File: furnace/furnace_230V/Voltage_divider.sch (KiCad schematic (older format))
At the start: 14 parts

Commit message: Add files via upload
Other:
- note added: "Input 230V voltage measurement circuit"
- note removed: "Input 230V voltage mesurement circuit"
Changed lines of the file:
@@
 $EndComp
 Text Notes 8850 2200 2    197  ~ 0
-Input 230V voltage mesurement circuit
+Input 230V voltage measurement circuit
 $Comp
 L Device:C C?

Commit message: Add files via upload
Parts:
- C15, C16, C17: renamed from C?; symbol Device:C -> furnace_230V-rescue:C-Device
- D4: renamed from D?; footprint (none) -> Diode_SMD:D_SMA-SMB_Universal_Handsoldering; symbol Device:D -> furnace_230V-rescue:D-Device
- D5: renamed from D?; symbol Diode:BAT54S -> furnace_230V-rescue:BAT54S-Diode
- D6: renamed from D?; footprint (none) -> Diode_SMD:D_SMA-SMB_Universal_Handsoldering; symbol Device:D_TVS -> furnace_230V-rescue:D_TVS-Device
- R10, R11, R12, R13, R14: renamed from R?; symbol Device:R -> furnace_230V-rescue:R-Device
- TP7, TP8, TP9: renamed from TP?; symbol Connector:TestPoint -> furnace_230V-rescue:TestPoint-Connector
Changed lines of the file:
@@
 $EndDescr
 $Comp
-L Device:R R?
+L furnace_230V-rescue:R-Device R?
 U 1 1 60AC3251
 P 4500 3650
 AR Path="/60AAE0B8/60AC3251" Ref="R?"  Part="1"
-AR Path="/60AAE4BD/60AC3251" Ref="R?"  Part="1"
-F 0 "R?" H 4570 3696 50  0000 L CNN
+AR Path="/60AAE4BD/60AC3251" Ref="R10"  Part="1"
+F 0 "R10" H 4570 3696 50  0000 L CNN
 F 1 "180k 0,25W 1%" H 4570 3605 50  0000 L CNN
 F 2 "" V 4430 3650 50  0001 C CNN
@@
 $EndComp
 $Comp
-L Device:R R?
+L furnace_230V-rescue:R-Device R?
 U 1 1 60AC39AB
 P 6150 4000
 AR Path="/60AAE0B8/60AC39AB" Ref="R?"  Part="1"
 AR Path="/60AAEC6C/60AC39AB" Ref="R?"  Part="1"
-AR Path="/60AAE4BD/60AC39AB" Ref="R?"  Part="1"
-F 0 "R?" V 6050 4000 50  0000 C CNN
+AR Path="/60AAE4BD/60AC39AB" Ref="R13"  Part="1"
+F 0 "R13" V 6050 4000 50  0000 C CNN
 F 1 "100" V 6250 4000 50  0000 C CNN
 F 2 "Resistor_SMD:R_0603_1608Metric_Pad1.05x0.95mm_HandSolder" V 6080 4000 50  0001 C CNN
@@
 $EndComp
 $Comp
-L Diode:BAT54S D?
+L furnace_230V-rescue:BAT54S-Diode D5
 U 1 1 60AC3BC9
 P 6700 3500
-F 0 "D?" V 6746 3588 50  0000 L CNN
+F 0 "D5" V 6746 3588 50  0000 L CNN
 F 1 "BAT54S" V 6655 3588 50  0000 L CNN
 F 2 "Package_TO_SOT_SMD:SOT-23" H 6775 3625 50  0001 L CNN
@@
 $EndComp
 $Comp
-L Device:D_TVS D?
+L furnace_230V-rescue:D_TVS-Device D6
 U 1 1 60AC5492
 P 7000 4150
-F 0 "D?" V 7050 4000 50  0000 C CNN
+F 0 "D6" V 7050 4000 50  0000 C CNN
 F 1 "D_TVS" V 6950 3950 50  0000 C CNN
-F 2 "" H 7000 4150 50  0001 C CNN
+F 2 "Diode_SMD:D_SMA-SMB_Universal_Handsoldering" H 7000 4150 50  0001 C CNN
 F 3 "~" H 7000 4150 50  0001 C CNN
 	1    7000 4150
@@
 $EndComp
 $Comp
-L Device:R R?
+L furnace_230V-rescue:R-Device R?
 U 1 1 60AC5A68
 P 7650 4000
 AR Path="/60AAE0B8/60AC5A68" Ref="R?"  Part="1"
 AR Path="/60AAEC6C/60AC5A68" Ref="R?"  Part="1"
-AR Path="/60AAE4BD/60AC5A68" Ref="R?"  Part="1"
-F 0 "R?" V 7550 4000 50  0000 C CNN
+AR Path="/60AAE4BD/60AC5A68" Ref="R14"  Part="1"
+F 0 "R14" V 7550 4000 50  0000 C CNN
 F 1 "1k" V 7750 4000 50  0000 C CNN
 F 2 "Resistor_SMD:R_0603_1608Metric_Pad1.05x0.95mm_HandSolder" V 7580 4000 50  0001 C CNN
@@
 $EndComp
 $Comp
-L Device:C C?
+L furnace_230V-rescue:C-Device C?
 U 1 1 60AC6425
 P 8000 4150
@@
 AR Path="/609CA6A8/60AE5653/60AC6425" Ref="C?"  Part="1"
 AR Path="/60AAC605/60AC6425" Ref="C?"  Part="1"
-AR Path="/60AAE4BD/60AC6425" Ref="C?"  Part="1"
-F 0 "C?" H 8115 4196 50  0000 L CNN
+AR Path="/60AAE4BD/60AC6425" Ref="C17"  Part="1"
+F 0 "C17" H 8115 4196 50  0000 L CNN
 F 1 "100" H 8115 4105 50  0000 L CNN
 F 2 "Capacitor_SMD:C_0603_1608Metric_Pad1.08x0.95mm_HandSolder" H 8038 4000 50  0001 C CNN
@@
 $EndComp
 $Comp
-L Connector:TestPoint TP?
+L furnace_230V-rescue:TestPoint-Connector TP?
 U 1 1 60ACD704
 P 5500 4000
@@
 AR Path="/609CA6A8/60AE5653/60ACD704" Ref="TP?"  Part="1"
 AR Path="/60AAC605/60ACD704" Ref="TP?"  Part="1"
-AR Path="/60AAE4BD/60ACD704" Ref="TP?"  Part="1"
-F 0 "TP?" H 5558 4118 50  0000 L CNN
+AR Path="/60AAE4BD/60ACD704" Ref="TP7"  Part="1"
+F 0 "TP7" H 5558 4118 50  0000 L CNN
 F 1 "TestPoint" H 5558 4027 50  0001 L CNN
 F 2 "" H 5700 4000 50  0001 C CNN
@@
 $EndComp
 $Comp
-L Connector:TestPoint TP?
+L furnace_230V-rescue:TestPoint-Connector TP?
 U 1 1 60ACD8BB
 P 5500 4500
@@
 AR Path="/609CA6A8/60AE5653/60ACD8BB" Ref="TP?"  Part="1"
 AR Path="/60AAC605/60ACD8BB" Ref="TP?"  Part="1"
-AR Path="/60AAE4BD/60ACD8BB" Ref="TP?"  Part="1"
-F 0 "TP?" H 5558 4618 50  0000 L CNN
+AR Path="/60AAE4BD/60ACD8BB" Ref="TP8"  Part="1"
+F 0 "TP8" H 5558 4618 50  0000 L CNN
 F 1 "TestPoint" H 5558 4527 50  0001 L CNN
 F 2 "" H 5700 4500 50  0001 C CNN
@@
 $EndComp
 $Comp
-L Connector:TestPoint TP?
+L furnace_230V-rescue:TestPoint-Connector TP?
 U 1 1 60ACDB72
 P 8500 4000
@@
 AR Path="/609CA6A8/60AE5653/60ACDB72" Ref="TP?"  Part="1"
 AR Path="/60AAC605/60ACDB72" Ref="TP?"  Part="1"
-AR Path="/60AAE4BD/60ACDB72" Ref="TP?"  Part="1"
-F 0 "TP?" H 8558 4118 50  0000 L CNN
+AR Path="/60AAE4BD/60ACDB72" Ref="TP9"  Part="1"
+F 0 "TP9" H 8558 4118 50  0000 L CNN
 F 1 "TestPoint" H 8558 4027 50  0001 L CNN
 F 2 "" H 8700 4000 50  0001 C CNN
@@
 Input 230V voltage measurement circuit
 $Comp
-L Device:C C?
+L furnace_230V-rescue:C-Device C?
 U 1 1 60B35196
 P 5000 4150
@@
 AR Path="/609CA6A8/60AE5653/60B35196" Ref="C?"  Part="1"
 AR Path="/60AAC605/60B35196" Ref="C?"  Part="1"
-AR Path="/60AAE4BD/60B35196" Ref="C?"  Part="1"
-F 0 "C?" H 5115 4196 50  0000 L CNN
+AR Path="/60AAE4BD/60B35196" Ref="C15"  Part="1"
+F 0 "C15" H 5115 4196 50  0000 L CNN
 F 1 "100" H 5115 4105 50  0000 L CNN
 F 2 "Capacitor_SMD:C_0603_1608Metric_Pad1.08x0.95mm_HandSolder" H 5038 4000 50  0001 C CNN
@@
 $EndComp
 $Comp
-L Device:R R?
+L furnace_230V-rescue:R-Device R?
 U 1 1 60B367EA
 P 4500 4150
@@
 AR Path="/60AAC605/60B367EA" Ref="R?"  Part="1"
 AR Path="/60AAE178/60B367EA" Ref="R?"  Part="1"
-AR Path="/60AAE4BD/60B367EA" Ref="R?"  Part="1"
-F 0 "R?" H 4570 4196 50  0000 L CNN
+AR Path="/60AAE4BD/60B367EA" Ref="R11"  Part="1"
+F 0 "R11" H 4570 4196 50  0000 L CNN
 F 1 "3,3k 1%" H 4570 4105 50  0000 L CNN
 F 2 "Resistor_SMD:R_0603_1608Metric_Pad0.98x0.95mm_HandSolder" V 4430 4150 50  0001 C CNN
@@
 $EndComp
 $Comp
-L Device:R R?
+L furnace_230V-rescue:R-Device R?
 U 1 1 60B376FC
 P 4500 4650
 AR Path="/60AAE0B8/60B376FC" Ref="R?"  Part="1"
-AR Path="/60AAE4BD/60B376FC" Ref="R?"  Part="1"
-F 0 "R?" H 4570 4696 50  0000 L CNN
+AR Path="/60AAE4BD/60B376FC" Ref="R12"  Part="1"
+F 0 "R12" H 4570 4696 50  0000 L CNN
 F 1 "180k 0,25W 1%" H 4570 4605 50  0000 L CNN
 F 2 "" V 4430 4650 50  0001 C CNN
@@
 $EndComp
 $Comp
-L Device:C C?
+L furnace_230V-rescue:C-Device C?
 U 1 1 60B3D4CA
 P 7300 3350
@@
 AR Path="/609CA6A8/60AE5653/60B3D4CA" Ref="C?"  Part="1"
 AR Path="/60AAC605/60B3D4CA" Ref="C?"  Part="1"
-AR Path="/60AAE4BD/60B3D4CA" Ref="C?"  Part="1"
-F 0 "C?" H 7415 3396 50  0000 L CNN
+AR Path="/60AAE4BD/60B3D4CA" Ref="C16"  Part="1"
+F 0 "C16" H 7415 3396 50  0000 L CNN
 F 1 "10u" H 7415 3305 50  0000 L CNN
 F 2 "Capacitor_SMD:C_0603_1608Metric_Pad1.08x0.95mm_HandSolder" H 7338 3200 50  0001 C CNN
@@
 $EndComp
 $Comp
-L Device:D D?
+L furnace_230V-rescue:D-Device D4
 U 1 1 60B3EF31
 P 3850 3500
-F 0 "D?" H 3850 3400 50  0000 C CNN
+F 0 "D4" H 3850 3400 50  0000 C CNN
 F 1 "ES1J" H 3850 3600 50  0000 C CNN
-F 2 "" H 3850 3500 50  0001 C CNN
+F 2 "Diode_SMD:D_SMA-SMB_Universal_Handsoldering" H 3850 3500 50  0001 C CNN
 F 3 "~" H 3850 3500 50  0001 C CNN
 	1    3850 3500

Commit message: Add files via upload
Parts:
- R10, R12: footprint (none) -> Resistor_THT:R_Axial_DIN0207_L6.3mm_D2.5mm_P10.16mm_Horizontal
- TP7, TP8, TP9: footprint (none) -> MountingHole:MountingHole_2.2mm_M2_DIN965_Pad_TopBottom
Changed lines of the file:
@@
 F 0 "R10" H 4570 3696 50  0000 L CNN
 F 1 "180k 0,25W 1%" H 4570 3605 50  0000 L CNN
-F 2 "" V 4430 3650 50  0001 C CNN
+F 2 "Resistor_THT:R_Axial_DIN0207_L6.3mm_D2.5mm_P10.16mm_Horizontal" V 4430 3650 50  0001 C CNN
 F 3 "~" H 4500 3650 50  0001 C CNN
 	1    4500 3650
@@
 F 0 "TP7" H 5558 4118 50  0000 L CNN
 F 1 "TestPoint" H 5558 4027 50  0001 L CNN
-F 2 "" H 5700 4000 50  0001 C CNN
+F 2 "MountingHole:MountingHole_2.2mm_M2_DIN965_Pad_TopBottom" H 5700 4000 50  0001 C CNN
 F 3 "~" H 5700 4000 50  0001 C CNN
 	1    5500 4000
@@
 F 0 "TP8" H 5558 4618 50  0000 L CNN
 F 1 "TestPoint" H 5558 4527 50  0001 L CNN
-F 2 "" H 5700 4500 50  0001 C CNN
+F 2 "MountingHole:MountingHole_2.2mm_M2_DIN965_Pad_TopBottom" H 5700 4500 50  0001 C CNN
 F 3 "~" H 5700 4500 50  0001 C CNN
 	1    5500 4500
@@
 F 0 "TP9" H 8558 4118 50  0000 L CNN
 F 1 "TestPoint" H 8558 4027 50  0001 L CNN
-F 2 "" H 8700 4000 50  0001 C CNN
+F 2 "MountingHole:MountingHole_2.2mm_M2_DIN965_Pad_TopBottom" H 8700 4000 50  0001 C CNN
 F 3 "~" H 8700 4000 50  0001 C CNN
 	1    8500 4000
@@
 F 0 "R12" H 4570 4696 50  0000 L CNN
 F 1 "180k 0,25W 1%" H 4570 4605 50  0000 L CNN
-F 2 "" V 4430 4650 50  0001 C CNN
+F 2 "Resistor_THT:R_Axial_DIN0207_L6.3mm_D2.5mm_P10.16mm_Horizontal" V 4430 4650 50  0001 C CNN
 F 3 "~" H 4500 4650 50  0001 C CNN
 	1    4500 4650

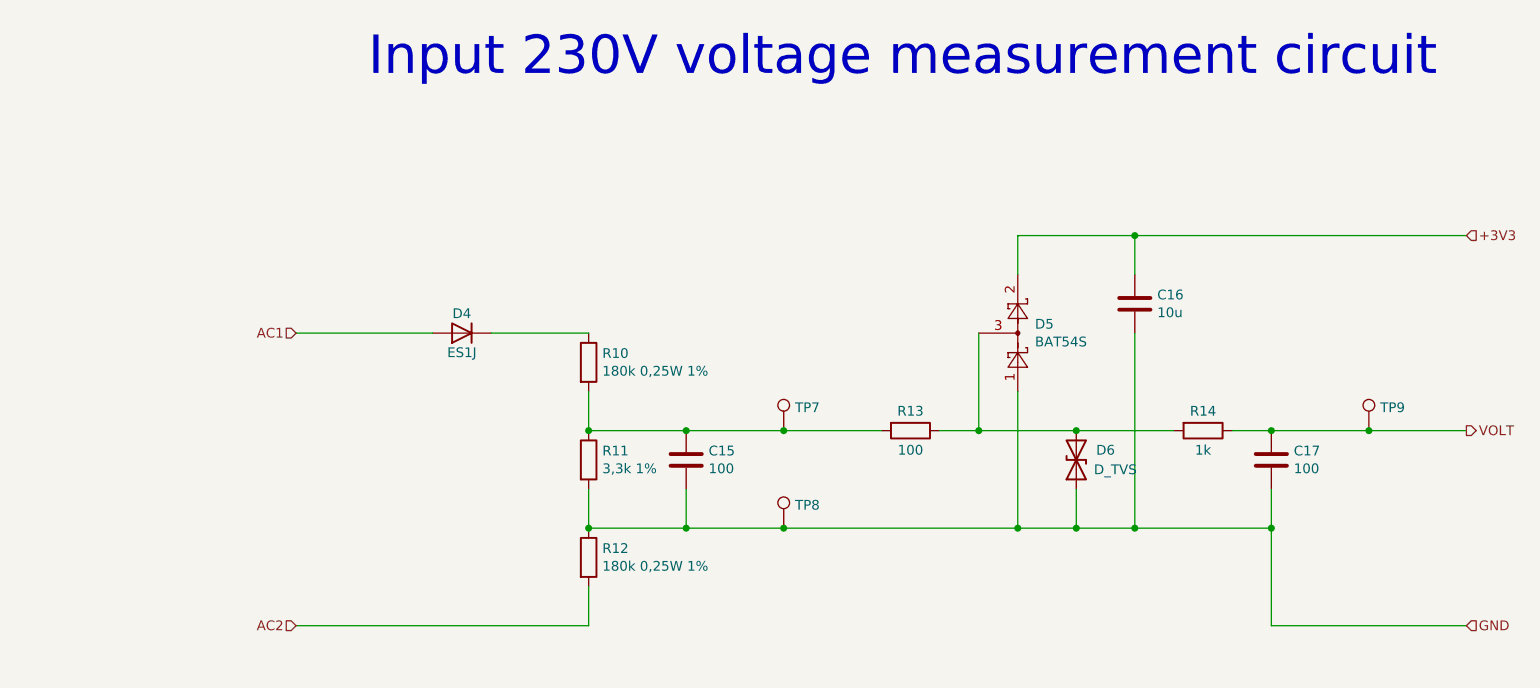
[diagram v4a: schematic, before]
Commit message: Add files via upload
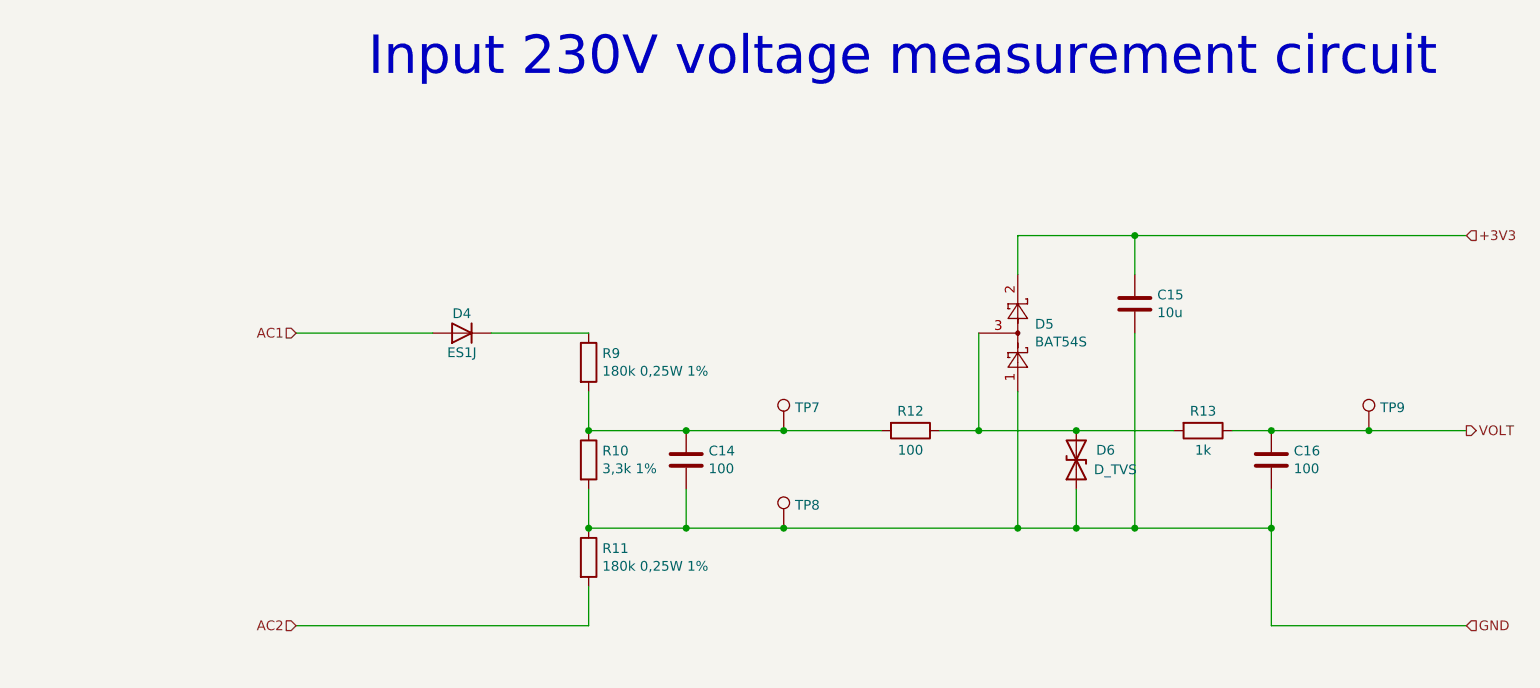
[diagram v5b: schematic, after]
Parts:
- C14: renamed from C15; footprint Capacitor_SMD:C_0603_1608Metric_Pad1.08x0.95mm_HandSolder -> Capacitor_SMD:C_0603_1608Metric_Pad1.05x0.95mm_HandSolder
- C15: renamed from C16; footprint Capacitor_SMD:C_0603_1608Metric_Pad1.08x0.95mm_HandSolder -> Capacitor_SMD:C_0603_1608Metric_Pad1.05x0.95mm_HandSolder
- C16: renamed from C17; footprint Capacitor_SMD:C_0603_1608Metric_Pad1.08x0.95mm_HandSolder -> Capacitor_SMD:C_0603_1608Metric_Pad1.05x0.95mm_HandSolder
- D4: footprint Diode_SMD:D_SMA-SMB_Universal_Handsoldering -> Diode_SMD:D_SMA_Handsoldering
- D6: footprint Diode_SMD:D_SMA-SMB_Universal_Handsoldering -> Diode_SMD:D_SMB_Handsoldering
- R10: renamed from R11; footprint Resistor_SMD:R_0603_1608Metric_Pad0.98x0.95mm_HandSolder -> Resistor_SMD:R_0603_1608Metric_Pad1.05x0.95mm_HandSolder
- TP7, TP8, TP9: footprint MountingHole:MountingHole_2.2mm_M2_DIN965_Pad_TopBottom -> furnace_230V:TP
- renumbered R12 to R11, R13 to R12, R14 to R13, R10 to R9
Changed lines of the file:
@@
 P 4500 3650
 AR Path="/60AAE0B8/60AC3251" Ref="R?"  Part="1"
-AR Path="/60AAE4BD/60AC3251" Ref="R10"  Part="1"
-F 0 "R10" H 4570 3696 50  0000 L CNN
+AR Path="/60AAE4BD/60AC3251" Ref="R9"  Part="1"
+F 0 "R9" H 4570 3696 50  0000 L CNN
 F 1 "180k 0,25W 1%" H 4570 3605 50  0000 L CNN
 F 2 "Resistor_THT:R_Axial_DIN0207_L6.3mm_D2.5mm_P10.16mm_Horizontal" V 4430 3650 50  0001 C CNN
@@
 AR Path="/60AAE0B8/60AC39AB" Ref="R?"  Part="1"
 AR Path="/60AAEC6C/60AC39AB" Ref="R?"  Part="1"
-AR Path="/60AAE4BD/60AC39AB" Ref="R13"  Part="1"
-F 0 "R13" V 6050 4000 50  0000 C CNN
+AR Path="/60AAE4BD/60AC39AB" Ref="R12"  Part="1"
+F 0 "R12" V 6050 4000 50  0000 C CNN
 F 1 "100" V 6250 4000 50  0000 C CNN
 F 2 "Resistor_SMD:R_0603_1608Metric_Pad1.05x0.95mm_HandSolder" V 6080 4000 50  0001 C CNN
@@
 F 0 "D6" V 7050 4000 50  0000 C CNN
 F 1 "D_TVS" V 6950 3950 50  0000 C CNN
-F 2 "Diode_SMD:D_SMA-SMB_Universal_Handsoldering" H 7000 4150 50  0001 C CNN
+F 2 "Diode_SMD:D_SMB_Handsoldering" H 7000 4150 50  0001 C CNN
 F 3 "~" H 7000 4150 50  0001 C CNN
 	1    7000 4150
@@
 AR Path="/60AAE0B8/60AC5A68" Ref="R?"  Part="1"
 AR Path="/60AAEC6C/60AC5A68" Ref="R?"  Part="1"
-AR Path="/60AAE4BD/60AC5A68" Ref="R14"  Part="1"
-F 0 "R14" V 7550 4000 50  0000 C CNN
+AR Path="/60AAE4BD/60AC5A68" Ref="R13"  Part="1"
+F 0 "R13" V 7550 4000 50  0000 C CNN
 F 1 "1k" V 7750 4000 50  0000 C CNN
 F 2 "Resistor_SMD:R_0603_1608Metric_Pad1.05x0.95mm_HandSolder" V 7580 4000 50  0001 C CNN
@@
 AR Path="/609CA6A8/60AE5653/60AC6425" Ref="C?"  Part="1"
 AR Path="/60AAC605/60AC6425" Ref="C?"  Part="1"
-AR Path="/60AAE4BD/60AC6425" Ref="C17"  Part="1"
-F 0 "C17" H 8115 4196 50  0000 L CNN
+AR Path="/60AAE4BD/60AC6425" Ref="C16"  Part="1"
+F 0 "C16" H 8115 4196 50  0000 L CNN
 F 1 "100" H 8115 4105 50  0000 L CNN
-F 2 "Capacitor_SMD:C_0603_1608Metric_Pad1.08x0.95mm_HandSolder" H 8038 4000 50  0001 C CNN
+F 2 "Capacitor_SMD:C_0603_1608Metric_Pad1.05x0.95mm_HandSolder" H 8038 4000 50  0001 C CNN
 F 3 "~" H 8000 4150 50  0001 C CNN
 	1    8000 4150
@@
 F 0 "TP7" H 5558 4118 50  0000 L CNN
 F 1 "TestPoint" H 5558 4027 50  0001 L CNN
-F 2 "MountingHole:MountingHole_2.2mm_M2_DIN965_Pad_TopBottom" H 5700 4000 50  0001 C CNN
+F 2 "furnace_230V:TP" H 5700 4000 50  0001 C CNN
 F 3 "~" H 5700 4000 50  0001 C CNN
 	1    5500 4000
@@
 F 0 "TP8" H 5558 4618 50  0000 L CNN
 F 1 "TestPoint" H 5558 4527 50  0001 L CNN
-F 2 "MountingHole:MountingHole_2.2mm_M2_DIN965_Pad_TopBottom" H 5700 4500 50  0001 C CNN
+F 2 "furnace_230V:TP" H 5700 4500 50  0001 C CNN
 F 3 "~" H 5700 4500 50  0001 C CNN
 	1    5500 4500
@@
 F 0 "TP9" H 8558 4118 50  0000 L CNN
 F 1 "TestPoint" H 8558 4027 50  0001 L CNN
-F 2 "MountingHole:MountingHole_2.2mm_M2_DIN965_Pad_TopBottom" H 8700 4000 50  0001 C CNN
+F 2 "furnace_230V:TP" H 8700 4000 50  0001 C CNN
 F 3 "~" H 8700 4000 50  0001 C CNN
 	1    8500 4000
@@
 AR Path="/609CA6A8/60AE5653/60B35196" Ref="C?"  Part="1"
 AR Path="/60AAC605/60B35196" Ref="C?"  Part="1"
-AR Path="/60AAE4BD/60B35196" Ref="C15"  Part="1"
-F 0 "C15" H 5115 4196 50  0000 L CNN
+AR Path="/60AAE4BD/60B35196" Ref="C14"  Part="1"
+F 0 "C14" H 5115 4196 50  0000 L CNN
 F 1 "100" H 5115 4105 50  0000 L CNN
-F 2 "Capacitor_SMD:C_0603_1608Metric_Pad1.08x0.95mm_HandSolder" H 5038 4000 50  0001 C CNN
+F 2 "Capacitor_SMD:C_0603_1608Metric_Pad1.05x0.95mm_HandSolder" H 5038 4000 50  0001 C CNN
 F 3 "~" H 5000 4150 50  0001 C CNN
 	1    5000 4150
@@
 AR Path="/60AAC605/60B367EA" Ref="R?"  Part="1"
 AR Path="/60AAE178/60B367EA" Ref="R?"  Part="1"
-AR Path="/60AAE4BD/60B367EA" Ref="R11"  Part="1"
-F 0 "R11" H 4570 4196 50  0000 L CNN
+AR Path="/60AAE4BD/60B367EA" Ref="R10"  Part="1"
+F 0 "R10" H 4570 4196 50  0000 L CNN
 F 1 "3,3k 1%" H 4570 4105 50  0000 L CNN
-F 2 "Resistor_SMD:R_0603_1608Metric_Pad0.98x0.95mm_HandSolder" V 4430 4150 50  0001 C CNN
+F 2 "Resistor_SMD:R_0603_1608Metric_Pad1.05x0.95mm_HandSolder" V 4430 4150 50  0001 C CNN
 F 3 "~" H 4500 4150 50  0001 C CNN
 	1    4500 4150
@@
 P 4500 4650
 AR Path="/60AAE0B8/60B376FC" Ref="R?"  Part="1"
-AR Path="/60AAE4BD/60B376FC" Ref="R12"  Part="1"
-F 0 "R12" H 4570 4696 50  0000 L CNN
+AR Path="/60AAE4BD/60B376FC" Ref="R11"  Part="1"
+F 0 "R11" H 4570 4696 50  0000 L CNN
 F 1 "180k 0,25W 1%" H 4570 4605 50  0000 L CNN
 F 2 "Resistor_THT:R_Axial_DIN0207_L6.3mm_D2.5mm_P10.16mm_Horizontal" V 4430 4650 50  0001 C CNN
@@
 AR Path="/609CA6A8/60AE5653/60B3D4CA" Ref="C?"  Part="1"
 AR Path="/60AAC605/60B3D4CA" Ref="C?"  Part="1"
-AR Path="/60AAE4BD/60B3D4CA" Ref="C16"  Part="1"
-F 0 "C16" H 7415 3396 50  0000 L CNN
+AR Path="/60AAE4BD/60B3D4CA" Ref="C15"  Part="1"
+F 0 "C15" H 7415 3396 50  0000 L CNN
 F 1 "10u" H 7415 3305 50  0000 L CNN
-F 2 "Capacitor_SMD:C_0603_1608Metric_Pad1.08x0.95mm_HandSolder" H 7338 3200 50  0001 C CNN
+F 2 "Capacitor_SMD:C_0603_1608Metric_Pad1.05x0.95mm_HandSolder" H 7338 3200 50  0001 C CNN
 F 3 "~" H 7300 3350 50  0001 C CNN
 	1    7300 3350
@@
 F 0 "D4" H 3850 3400 50  0000 C CNN
 F 1 "ES1J" H 3850 3600 50  0000 C CNN
-F 2 "Diode_SMD:D_SMA-SMB_Universal_Handsoldering" H 3850 3500 50  0001 C CNN
+F 2 "Diode_SMD:D_SMA_Handsoldering" H 3850 3500 50  0001 C CNN
 F 3 "~" H 3850 3500 50  0001 C CNN
 	1    3850 3500
